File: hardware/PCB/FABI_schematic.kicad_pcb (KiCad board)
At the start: 2 copper layers, 81 x 55 mm, 51 parts, among them J1 AudioJack3_Ground, J10 Conn_01x03_Male, J11 display_connector_91601-304LF, J11_GND1 Conn_01x01_Male, J11_VDD1 Conn_01x01_Male, J11_data1 Conn_01x01_Male, J2 AudioJack3_Ground, J3 AudioJack3_Ground, J4 AudioJack3_Ground, J5 AudioJack3_Ground, J6 AudioJack3_Ground, J7 AudioJack3_Ground, J8 AudioJack3_Ground, J9 Conn_02x05_Odd_Even, U1 MPXV7007GP, U2 ProMicro

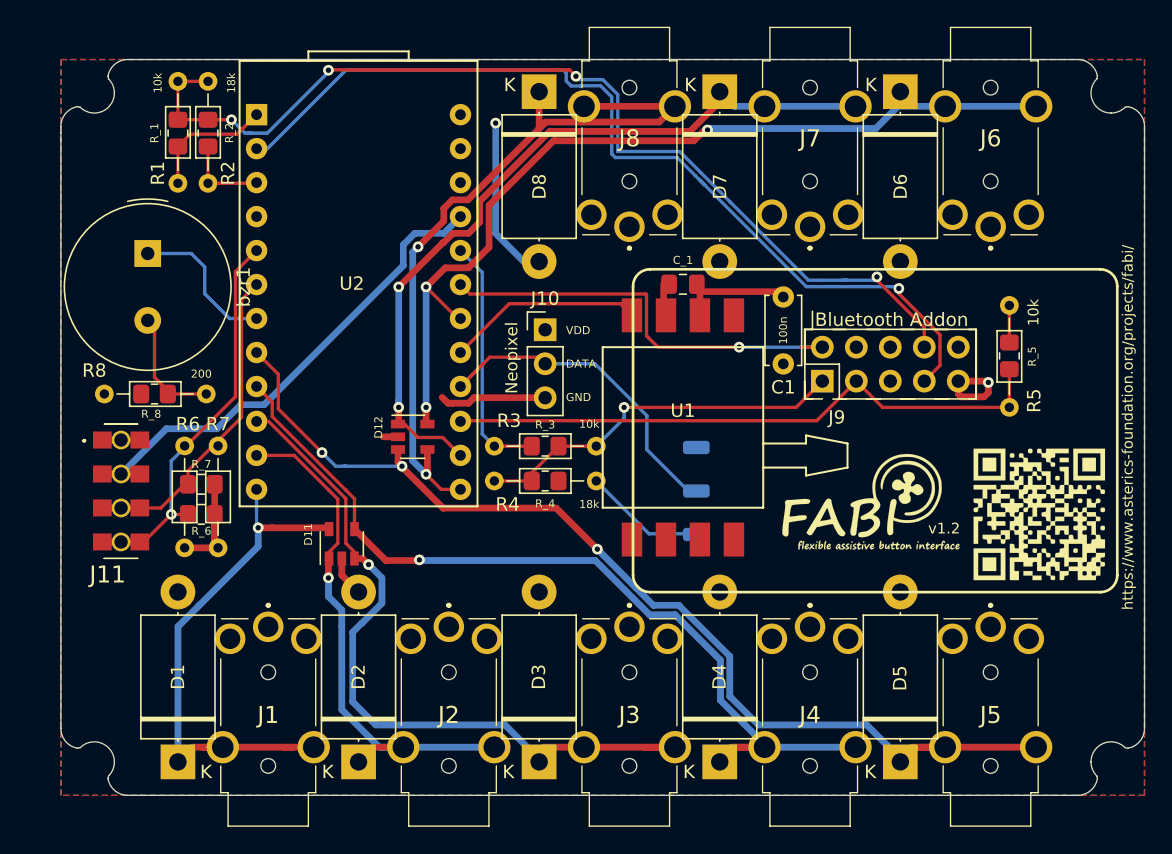
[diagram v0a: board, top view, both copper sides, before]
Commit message: First PCB draft of FABI3
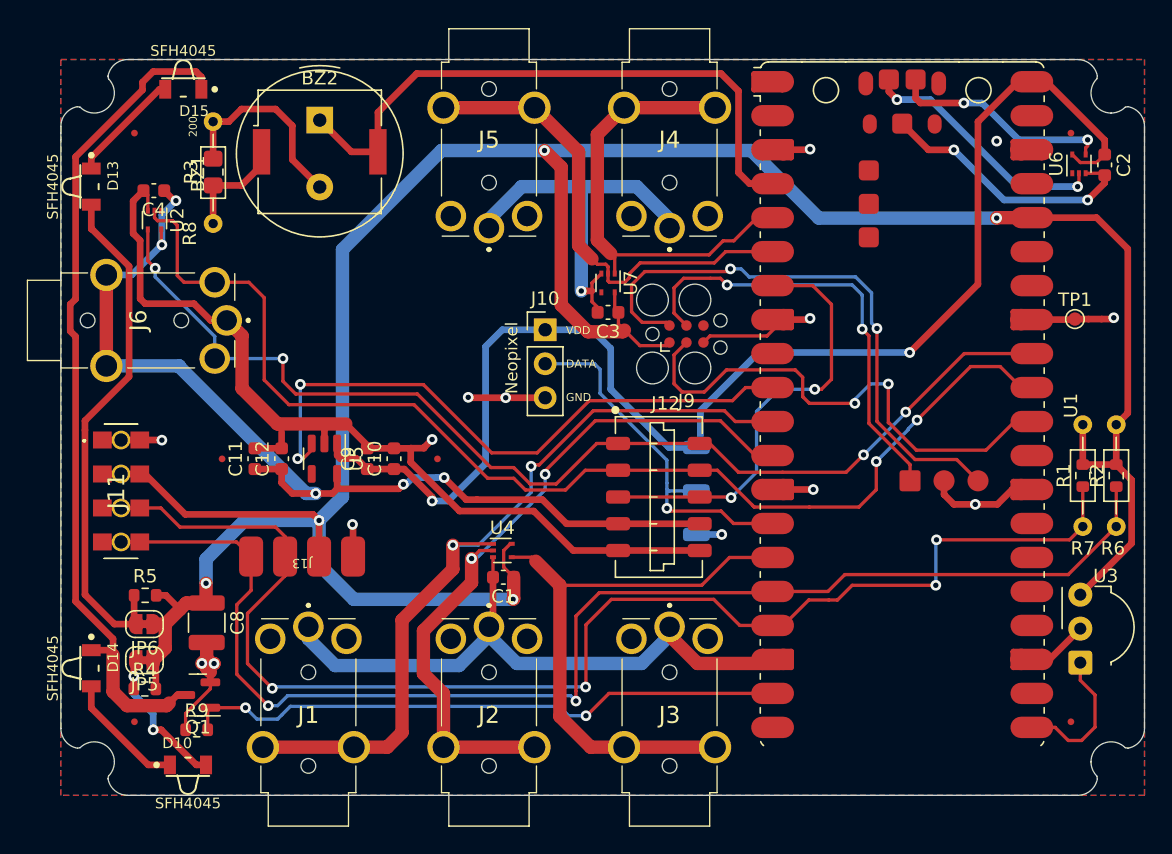
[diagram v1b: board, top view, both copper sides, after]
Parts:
- removed C_1: 100n, Capacitor_SMD:C_0805_2012Metric_Pad1.18x1.45mm_HandSolder
- removed D1, D2, D3, D4, D5, D6, D7, D8: P6KE6.8A, Diode_THT:D_DO-201AE_P12.70mm_Horizontal
- removed D11, D12: SP0504BAHT, Package_TO_SOT_SMD:SOT-23-5
- removed G*** (x2): LOGO, FABI_customLibs:QR_FABI_ProjectPage
- removed G***: LOGO, Logos:fabi_15x8
- removed G***: LOGO, FABI_customLibs:FABI_Logo_s
- removed G***: LOGO, FABI_customLibs:FH_logo_m
- removed J7, J8: AudioJack3_Ground, FABI_customLibs:FC68125
- removed REF**: ESP32_Addon, FABI_customLibs:ESP32_Addon
- removed R_1, R_3, R_5, R_6, R_7: 10k, Resistor_SMD:R_0805_2012Metric_Pad1.20x1.40mm_HandSolder
- removed R_2, R_4: 18k, Resistor_SMD:R_0805_2012Metric_Pad1.20x1.40mm_HandSolder
- removed R_8: 200, Resistor_SMD:R_0805_2012Metric_Pad1.20x1.40mm_HandSolder
- removed bzr1: Buzzer, Buzzer_Beeper:Buzzer_TDK_PS1240P02BT_D12.2mm_H6.5mm
- added BZ1: Buzzer, Buzzer_Beeper:Buzzer_TDK_PS1240P02BT_D12.2mm_H6.5mm, F.Cu at (106.6, 88.4)
- added BZ2: PKMCS0909E4000, Buzzer_Beeper:Buzzer_Murata_PKMCS0909E, F.Cu at (106.6, 90.7)
- added C10: 100n, Capacitor_SMD:C_0603_1608Metric, F.Cu at (112.1, 113.7)
- added C11: 100n, Capacitor_SMD:C_0603_1608Metric, F.Cu at (101.7, 113.7)
- added C12: 1uF / >6.3V / X7R, Capacitor_SMD:C_0603_1608Metric, F.Cu at (103.7, 113.7)
- added C2: 100n, Capacitor_SMD:C_0603_1608Metric, F.Cu at (165.3, 91.7)
- added C3: 100n, Capacitor_SMD:C_0603_1608Metric, F.Cu at (128.1, 102.7)
- added C4: 100n, Capacitor_SMD:C_0603_1608Metric, F.Cu at (94.2, 93.6)
- added C8: 100uF/6.3V, Capacitor_SMD:C_1210_3225Metric, F.Cu at (98.1, 125.9)
- added C9: 1uF / >6.3V / X7R, Capacitor_SMD:C_0603_1608Metric, F.Cu at (110.1, 113.7)
- added D10: SFH4045, FLipMouse:SFH4045N, F.Cu at (96.7, 137.3)
- added D13: SFH4045, FLipMouse:SFH4045N, F.Cu at (88.7, 93.3)
- added D14: SFH4045, FLipMouse:SFH4045N, F.Cu at (88.7, 129.3)
- added D15: SFH4045, FLipMouse:SFH4045N, F.Cu at (96.4, 85.3)
- added FID10: Fiducial, Fiducial:Fiducial_0.5mm_Mask1mm, F.Cu at (162.7, 89.3)
- added FID11: Fiducial, Fiducial:Fiducial_0.5mm_Mask1mm, F.Cu at (99.3, 113.7)
- added FID12: Fiducial, Fiducial:Fiducial_0.5mm_Mask1mm, F.Cu at (115.4, 113.7)
- added FID7: Fiducial, Fiducial:Fiducial_0.5mm_Mask1mm, F.Cu at (92.7, 89.3)
- added FID8: Fiducial, Fiducial:Fiducial_0.5mm_Mask1mm, F.Cu at (92.7, 133.3)
- added FID9: Fiducial, Fiducial:Fiducial_0.5mm_Mask1mm, F.Cu at (162.7, 133.3)
- added J12: 009159005551906, FLipMouse:009159005551906, F.Cu at (131.9, 116.5)
- added J13: Conn_01x04_Male, FLipMouse:pressure_sensor, F.Cu at (105.3, 121.0)
- added JP5: SolderJumper_2_Bridged, Jumper:SolderJumper-2_P1.3mm_Bridged_RoundedPad1.0x1.5mm, F.Cu at (93.5, 128.7)
- added JP6: SolderJumper_2_Bridged, Jumper:SolderJumper-2_P1.3mm_Bridged_RoundedPad1.0x1.5mm, F.Cu at (93.5, 126.0)
- added LOGO5: Logo_FABI, FABI:FABI_Logo_s, B.Cu at (152.1, 94.6)
- added LOGO6: Logo_KiCAD, Symbol:KiCad-Logo_5mm_SilkScreen, B.Cu at (119.7, 118.0)
- added LOGO7: Logo_CE, Symbol:CE-Logo_8.5x6mm_SilkScreen, B.Cu at (147.5, 128.3)
- added LOGO8: Logo_WEEE, Symbol:WEEE-Logo_5.6x8mm_SilkScreen, B.Cu at (155.3, 127.8)
- added NT1: NetTie_2, NetTie:NetTie-2_SMD_Pad0.5mm, F.Cu at (164.5, 103.2)
- added NT2: NetTie_2, NetTie:NetTie-2_SMD_Pad0.5mm, F.Cu at (113.9, 112.9)
- added Q1: BSS806, Package_TO_SOT_SMD:SOT-23, F.Cu at (97.5, 131.3)
- added R9: 4k7, Resistor_SMD:R_0603_1608Metric, F.Cu at (97.4, 133.9)
- added TP1: TestPoint, TestPoint:TestPoint_Pad_D1.0mm, F.Cu at (163.0, 103.2)
- added U3: TSOP4838, OptoDevice:Vishay_MOLD-3Pin, F.Cu at (163.4, 128.9)
- added U4: TPD3E001DRLR, Package_TO_SOT_SMD:SOT-553, F.Cu at (120.2, 120.5)
- added U5: MIC5504-3.3YM5, Package_TO_SOT_SMD:SOT-23-5, F.Cu at (106.9, 113.7)
- added U6: TPD3E001DRLR, Package_TO_SOT_SMD:SOT-553, F.Cu at (163.3, 91.6)
- added U7: TPD3E001DRLR, Package_TO_SOT_SMD:SOT-553, F.Cu at (128.1, 100.5)
- C1: footprint Capacitor_THT:C_Disc_D5.0mm_W2.5mm_P5.00mm -> Capacitor_SMD:C_0603_1608Metric
- J1, J2, J3, J4, J5, J6: footprint FABI_customLibs:FC68125 -> FABI:FC68125
- J11: footprint FABI_customLibs:91601304LF -> FABI:91601304LF
- J9: value Conn_02x05_Odd_Even -> Conn_ARM_SWD_TagConnect_TC2030; footprint Connector_PinHeader_2.54mm:PinHeader_2x05_P2.54mm_Vertical -> Connector:Tag-Connect_TC2030-IDC-FP_2x03_P1.27mm_Vertical
- R1: value 10k -> 4k7; footprint Resistor_THT:R_Axial_DIN0204_L3.6mm_D1.6mm_P7.62mm_Horizontal -> Resistor_SMD:R_0603_1608Metric
- R2: value 18k -> 4k7; footprint Resistor_THT:R_Axial_DIN0204_L3.6mm_D1.6mm_P7.62mm_Horizontal -> Resistor_SMD:R_0603_1608Metric
- R3: value 10k -> 200; footprint Resistor_THT:R_Axial_DIN0204_L3.6mm_D1.6mm_P7.62mm_Horizontal -> Resistor_SMD:R_0805_2012Metric_Pad1.20x1.40mm_HandSolder
- R4: value 18k -> DNP; footprint Resistor_THT:R_Axial_DIN0204_L3.6mm_D1.6mm_P7.62mm_Horizontal -> Resistor_SMD:R_0603_1608Metric
- R5: value 10k -> DNP; footprint Resistor_THT:R_Axial_DIN0204_L3.6mm_D1.6mm_P7.62mm_Horizontal -> Resistor_SMD:R_0603_1608Metric
- U1: value MPXV7007GP -> RaspberryPi_Pico_W_SecondaryPins; footprint MPXV7007GP:MPXV7007GP -> Module_RaspberryPi_Pico:RaspberryPi_Pico_W_SMD
- U2: value ProMicro -> TPD3E001DRLR; footprint FABI_customLibs:ProMicro -> Package_TO_SOT_SMD:SOT-553
- moved R2 74.0 mm to (166.1, 114.9), turned to 90 degrees
- moved R1 71.1 mm to (163.6, 114.9)
- moved R6 70.2 mm to (166.1, 111.1), turned to -90 degrees
- moved R5 66.1 mm to (93.5, 123.9), turned to 0 degrees
- moved R7 65.3 mm to (163.6, 111.1), turned to -90 degrees
- moved J6 65.1 mm to (93.0, 103.3), turned to 90 degrees
- moved J5 57.1 mm to (119.2, 89.8), turned to 0 degrees
- moved J4 44.3 mm to (132.7, 89.8), turned to 0 degrees
- moved R4 30.4 mm to (93.5, 130.9)
- moved C1 29.6 mm to (120.3, 122.5), turned to 180 degrees
- moved R3 29.4 mm to (98.6, 92.3), turned to 90 degrees
- moved U1 16.5 mm to (150.1, 109.6), turned to 0 degrees
- moved U2 16.0 mm to (94.2, 95.8)
- moved R8 15.1 mm to (98.6, 96.1), turned to 90 degrees
- moved J9 10.8 mm to (134.0, 104.4), turned to 0 degrees
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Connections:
- J1 pad 2R: Net-(J1-Pad2R) -> unconnected-(J1-Pad2R)
- J1 pad 3T: AUX_1 -> /BUTTON1
- J1 pad 6SR: Net-(J1-Pad6SR) -> unconnected-(J1-Pad6SR)
- J10 pad 1: VCC -> VBUS
- J10 pad 2: NEOPIXEL -> /NEOPIXEL
- J11 pad 5: SCL -> /SCL_INT
- J11 pad 7: SDA -> /SDA_INT
- J11_VDD1 pad 1: VCC -> VBUS
- J11_data1 pad 1: NEOPIXEL -> /NEOPIXEL
- J2 pad 2R: Net-(J2-Pad2R) -> unconnected-(J2-Pad2R)
- J2 pad 3T: AUX_2 -> /BUTTON2
- J2 pad 6SR: Net-(J2-Pad6SR) -> unconnected-(J2-Pad6SR)
- J3 pad 2R: Net-(J3-Pad2R) -> unconnected-(J3-Pad2R)
- J3 pad 3T: AUX_3 -> /BUTTON3
- J3 pad 6SR: Net-(J3-Pad6SR) -> unconnected-(J3-Pad6SR)
- J4 pad 2R: Net-(J4-Pad2R) -> unconnected-(J4-Pad2R)
- J4 pad 3T: AUX_4 -> /BUTTON4
- J4 pad 6SR: Net-(J4-Pad6SR) -> unconnected-(J4-Pad6SR)
- J5 pad 2R: Net-(J5-Pad2R) -> unconnected-(J5-Pad2R)
- J5 pad 3T: AUX_5 -> /BUTTON5
- J5 pad 6SR: Net-(J5-Pad6SR) -> unconnected-(J5-Pad6SR)
- J6 pad 1S: GND -> GNDA
- J6 pad 2R: Net-(J6-Pad2R) -> /SCL
- J6 pad 3T: AUX_6 -> +3.3VADC
- J6 pad 6SR: Net-(J6-Pad6SR) -> /SDA
- J9 pad 1: ESP_AddOn_Pin1 -> VCC
- J9 pad 2: AddOn_Pin2 -> Net-(J9-SWDIO)
- J9 pad 3: AddOn_Pin3 -> /RESET
- J9 pad 4: Net-(J9-Pad4) -> Net-(J9-SWCLK)
- J9 pad 5: Net-(J9-Pad5) -> GND
- J9 pad 6: GND -> unconnected-(J9-SWO-Pad6)
- R1 pad 1: A_TX -> /SCL_INT
- R1 pad 2: ESP_RX -> VCC
- R2 pad 1: ESP_RX -> /SDA_INT
- R2 pad 2: GND -> VCC
- R3 pad 1: AddOn_Pin1 -> GND
- R3 pad 2: ESP_AddOn_Pin1 -> Net-(BZ1-+)
- R4 pad 1: ESP_AddOn_Pin1 -> Net-(D10-A)
- R4 pad 2: GND -> VCC
- R5 pad 1: AddOn_Pin3 -> Net-(D13-A)
- R5 pad 2: GND -> VCC
- R6 pad 2: SDA -> /SDA_INT
- R7 pad 2: SCL -> /SCL_INT
- R8 pad 2: Net-(R8-Pad2) -> Net-(BZ1-+)
- U1 pad 1: Net-(U1-Pad1) -> unconnected-(U1-GPIO0-Pad1)
- U1 pad 2: VCC -> unconnected-(U1-GPIO1-Pad2)
- U1 pad 4: MPX -> /BUZZER
- U1 pad 5: Net-(U1-Pad5) -> /BUTTON4
- U1 pad 6: Net-(U1-Pad6) -> /BUTTON5
- U1 pad 7: Net-(U1-Pad7) -> /MPRLS_DRDY_RES
- U1 pad 8: Net-(U1-Pad8) -> GND
- U2 pad 1: A_TX -> unconnected-(U2-IO1-Pad1)
- U2 pad 2: A_RX -> /SDA
- U2 pad 3: GND -> GNDA
- U2 pad 4: GND -> /SCL
- U2 pad 5: SDA -> +3.3VADC
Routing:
- net VCC: track 62.6 -> 213.4 mm, vias 1 -> 5
- net /SCL_INT: track 0.00 -> 105.7 mm, vias 0 -> 4
- net VBUS: track 0.00 -> 101.4 mm, vias 0 -> 2
- net /SDA_INT: track 0.00 -> 100.1 mm, vias 0 -> 2
- net /SDA: track 0.00 -> 87.5 mm, vias 0 -> 2
- net GND: track 50.1 -> 136.9 mm, vias 1 -> 15
- net /SCL: track 0.00 -> 82.7 mm, vias 0 -> 4
- net AUX_5: track 80.7 -> 0.00 mm, vias 3 -> 0
- net ESP_RX: track 78.4 -> 0.00 mm, vias 4 -> 0
- net +3.3VADC: track 0.00 -> 75.2 mm, vias 0 -> 5
- net A_RX: track 69.6 -> 0.00 mm, vias 1 -> 0
- net GNDA: track 0.00 -> 69.0 mm
- net AUX_6: track 68.4 -> 0.00 mm, vias 3 -> 0
- net AUX_4: track 67.7 -> 0.00 mm, vias 1 -> 0
- net Net-(D14-K): track 0.00 -> 62.9 mm
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- added copper zone on B.Cu, net GND
- removed copper zone on B.Cu, net VCC
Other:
- board text added: "+5V"
- board text added: "FABI - Flexible Assistive Button Interface AsTeRICS Foundation / UAS Technikum Wien office@asterics-foundation.org Benjamin Aigner"
- board text added: "https://www.asterics-foundation.org/projects/fabi/ https://github.com/asterics/fabi"
- board text added: "v3.0"
- board text removed: "Bluetooth Addon"
- board text removed: "FABI - Flexible Assistive Button Interface AsTeRICS Foundation / UAS Technikum Wien office@asterics-foundation.org Benjamin Aigner, Andreas Fußthaler, Christoph Veigl"
- board text removed: "https://www.asterics-foundation.org/projects/fabi/"
- board text removed: "v1.2"
